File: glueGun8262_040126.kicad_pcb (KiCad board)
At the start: 2 copper layers, 104.9 x 99.1 mm, 73 parts, among them CN1 KF243-5.0-2P, CN2 KF243-5.0-2P, CN3 KF243-5.0-2P, CN4 KF243-5.0-2P, CN5 KF243-5.0-2P, CN6 KF243-5.0-2P, CN7 KF243-5.0-2P, CN9 KF243-5.0-4P, Q1 SQM120P10-10m1L, U1 DRV8262DDWR, U10 INA240A2DR, U11 INA240A2DR, U2 DRV8262DDWR, U3 ESP32-S3-DEVKITC-1-N8R8, U5 6N137, U6 INA240A2DR, U7 INA240A2DR, U8 K7805-1000R3_C2992391, U9 TLP281-4(GB-TP,J,F

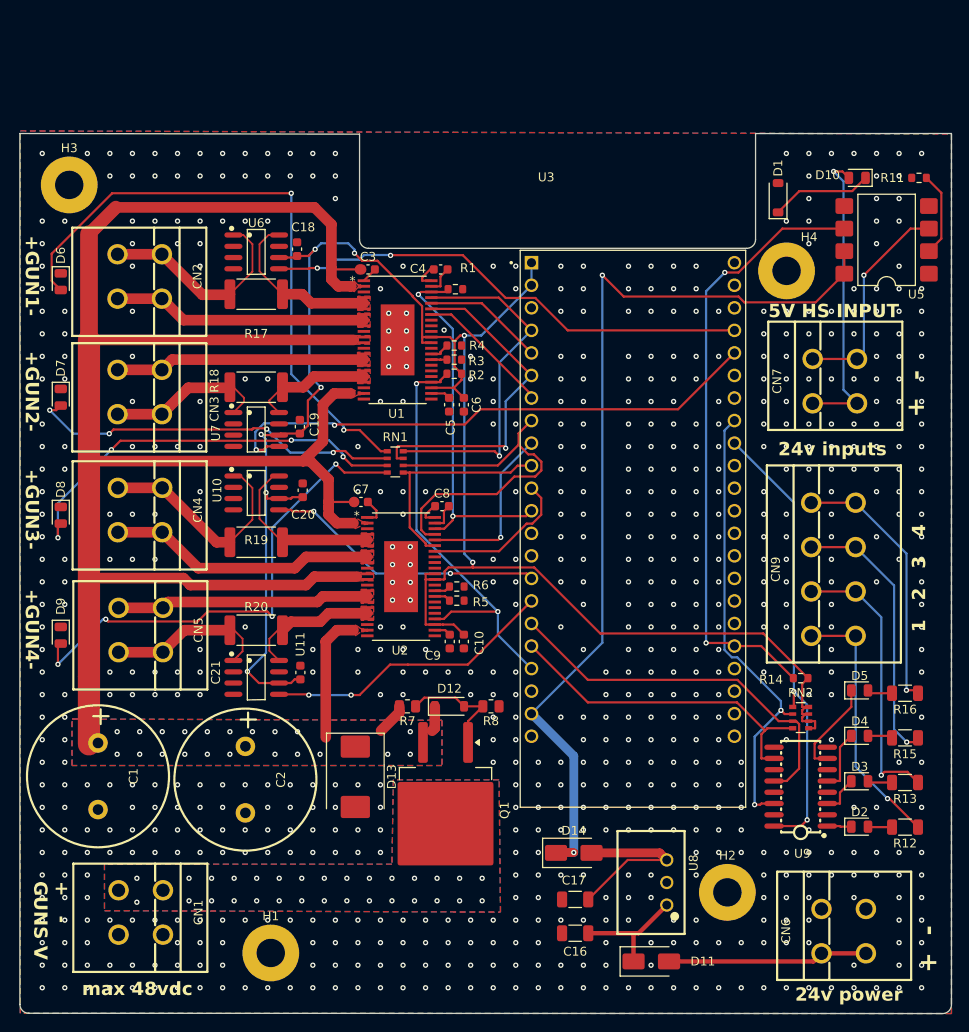
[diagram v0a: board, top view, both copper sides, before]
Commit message: redesigned before freerouting
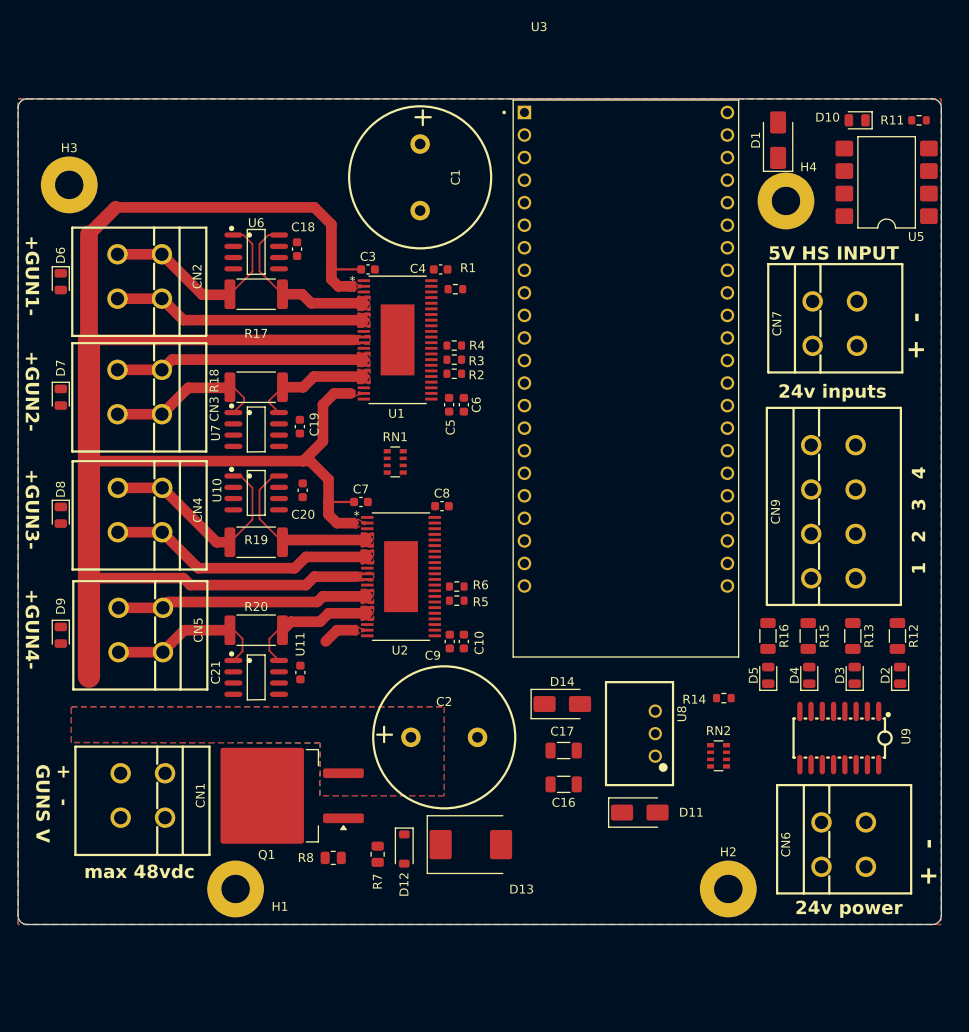
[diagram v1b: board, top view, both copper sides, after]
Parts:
- D1: value D_Schottky_AKK -> reverse protection; footprint Diode_SMD:D_SOD-123 -> Diode_SMD:D_SMA
- moved C1 76.6 mm to (151.3, 48.8)
- moved R8 24.6 mm to (141.5, 125.5), turned to 0 degrees
- moved C2 22.9 mm to (154.0, 111.9), turned to 0 degrees
- moved R12 21.5 mm to (205.1, 100.5), turned to -90 degrees
- moved Q1 19.2 mm to (135.0, 118.5), turned to 180 degrees
- moved D2 17.6 mm to (205.4, 104.9), turned to 90 degrees
- moved R13 17.5 mm to (200.0, 100.5), turned to -90 degrees
- moved R7 17.0 mm to (146.5, 125.1), turned to 90 degrees
- moved U3 16.9 mm to (174.5, 71.5)
- moved D12 16.9 mm to (149.5, 124.5), turned to -90 degrees
- moved C16 16.8 mm to (167.5, 117.2)
- moved C17 16.8 mm to (167.5, 113.4)
- moved U8 16.8 mm to (177.8, 111.5)
- moved D11 16.8 mm to (176.0, 120.4)
- moved D14 16.8 mm to (167.3, 108.2)
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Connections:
- D1 pad 1: Net-(D1-A) -> Net-(D1-K)
- D1 pad 2: unconnected-(D1-K-Pad2) -> Net-(D1-A)
- R11 pad 1: Net-(D1-K-Pad3) -> Net-(D1-K)
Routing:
- net +3V3: track 216.9 -> 0.00 mm, vias 8 -> 0
- net +5V: track 104.7 -> 0.00 mm, vias 2 -> 0
- net /Input_0_5v: track 69.6 -> 0.00 mm, vias 2 -> 0
- net Net-(D6-A): track 69.3 -> 0.00 mm, vias 2 -> 0
- net /Gun2Vref: track 62.6 -> 0.00 mm, vias 2 -> 0
- net Net-(D9-A): track 55.8 -> 0.00 mm, vias 4 -> 0
- net /Gun1Vref: track 55.5 -> 0.00 mm, vias 2 -> 0
- net /Input_2_24v: track 51.7 -> 0.00 mm, vias 2 -> 0
- net /Input_1_24v: track 51.7 -> 0.00 mm, vias 2 -> 0
- net /nFAULT: track 48.9 -> 0.00 mm, vias 2 -> 0
- net Net-(D8-A): track 47.0 -> 0.00 mm, vias 4 -> 0
- net /Input_3_24v: track 43.3 -> 0.00 mm
- net Net-(D7-A): track 42.4 -> 0.00 mm, vias 4 -> 0
- net /nSLEEP: track 42.2 -> 0.00 mm, vias 2 -> 0
- net /U2_IN1: track 41.1 -> 0.00 mm
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- removed copper zone on B.Cu, net Net-(Q1-D)
- removed copper zone on F.Cu, net Net-(Q1-D)
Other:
- board size 104.9 x 99.1 mm -> 104 x 93 mm
